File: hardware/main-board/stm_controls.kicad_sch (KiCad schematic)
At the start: 24 parts, among them SW1 SW_SPST, U1 74HC164, U10 MT8816AF1, U11 MT8816AF1, U12 MT8816AF1, U13 AD5263BRUZ200, U14 AD5263BRUZ200, U15 AD5263BRUZ200, U16 AD5263BRUZ200, U17 AD5263BRUZ200, U18 AD5263BRUZ200, U19 AD5263BRUZ200, U2 74HC164, U20 AD5263BRUZ200, U22 STM32F091RCTx, U23 FT232RL, U3 74HC164, U4 MT8816AF1, U5 MT8816AF1, U6 MT8816AF1, U7 MT8816AF1, U8 MT8816AF1, U9 MT8816AF1

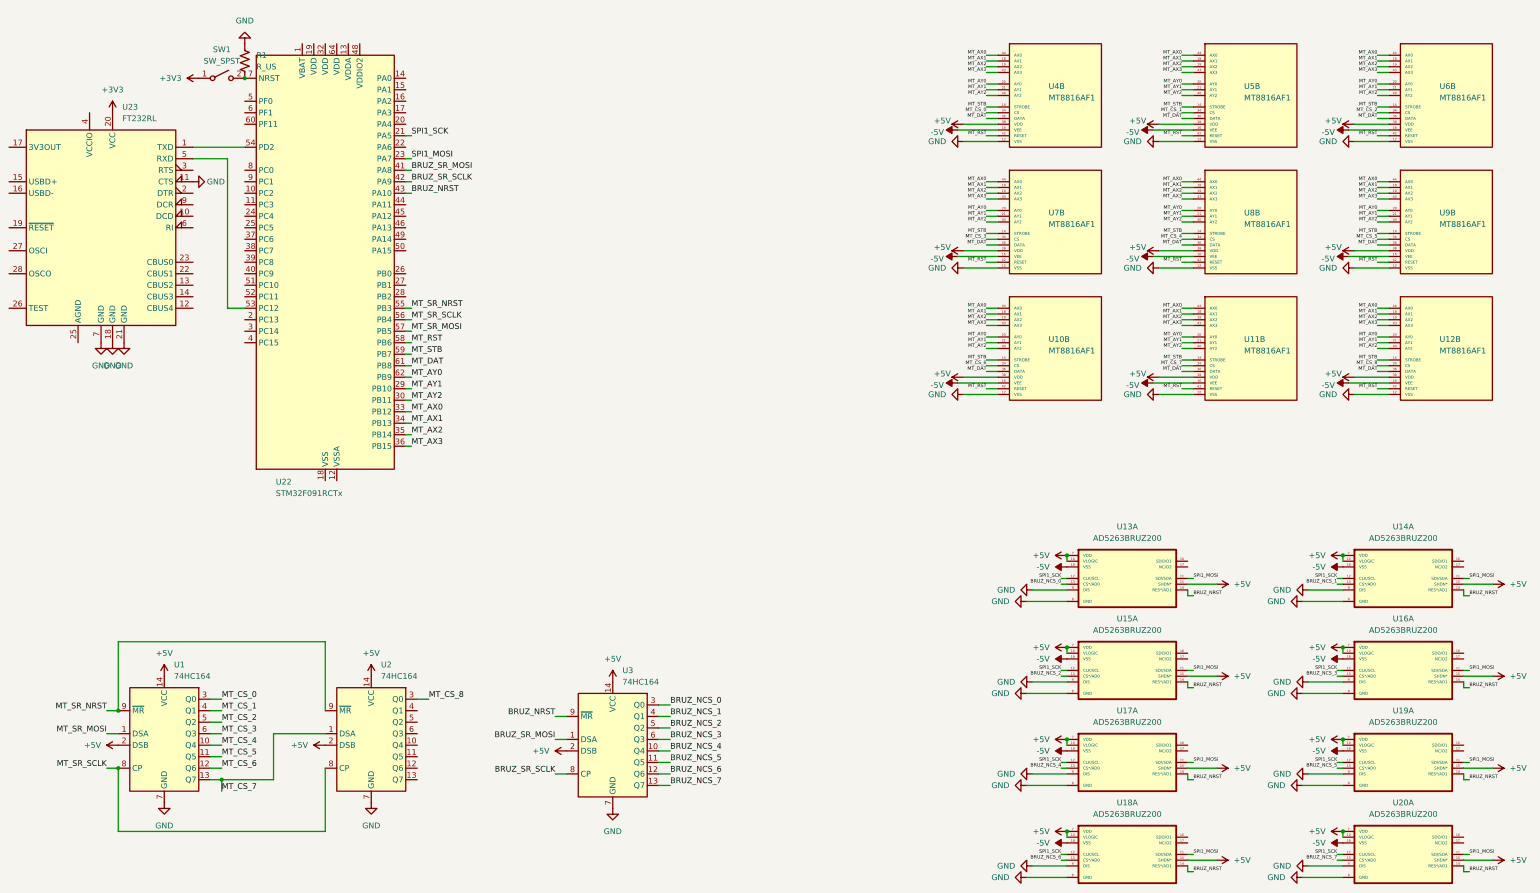
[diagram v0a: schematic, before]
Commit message: God is Real, God is Real, Im not kidding this time I wouldn't joke about this
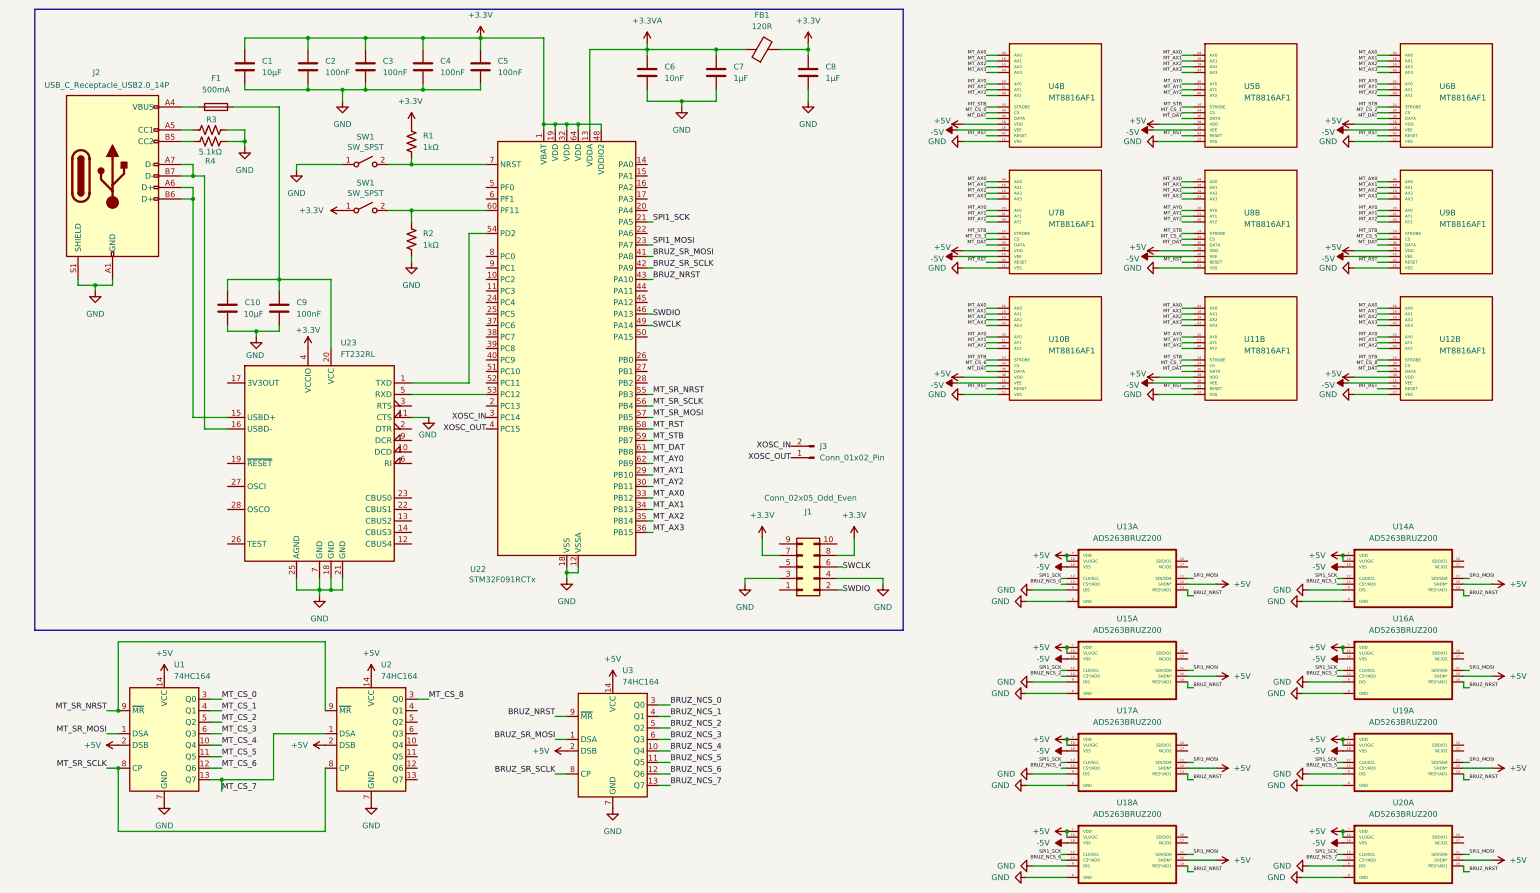
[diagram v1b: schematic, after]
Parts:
- added C1, C10: 10µF, symbol Device:C
- added C2, C3, C4, C5, C9: 100nF, symbol Device:C
- added C6: 10nF, symbol Device:C
- added C7, C8: 1µF, symbol Device:C
- added F1: 500mA, symbol Device:Fuse
- added FB1: 120R, symbol Device:FerriteBead
- added J1: Conn_02x05_Odd_Even, symbol Connector_Generic:Conn_02x05_Odd_Even
- added J2: USB_C_Receptacle_USB2.0_14P, symbol Connector:USB_C_Receptacle_USB2.0_14P
- added J3: Conn_01x02_Pin, symbol Connector:Conn_01x02_Pin
- added R2: 1kΩ, symbol Device:R_US
- added R3: 5.1kΩ, symbol Device:R_US
- added R4: R_US, symbol Device:R_US
- added SW1: SW_SPST, symbol Switch:SW_SPST
- R1: value R_US -> 1kΩ
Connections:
- net GND: now also SW1.1 (A), U22.12 (VSSA), U22.18 (VSS), U22.31 (VSS), U22.47 (VSS), U22.63 (VSS), U23.25 (AGND), C1.2, C10.2, C2.2, C3.2, C4.2, C5.2, C6.2, C7.2, C8.2, C9.2, J1.3 (Pin_3), J1.4 (Pin_4), J2.A1 (GND), J2.A12 (GND), J2.B1 (GND), J2.B12 (GND), J2.S1 (SHIELD), R2.2, R3.2, R4.2; no longer R1.1
- net at U23.15 (USBD+): now also J2.A6 (D+), J2.B6 (D+)
- net at U23.16 (USBD-): now also J2.A7 (D-), J2.B7 (D-)
- net +3.3V: now reaches U23.4 (VCCIO)
- net +3.3V: now also R1.1, U22.1 (VBAT), U22.19 (VDD), U22.32 (VDD), U22.48 (VDDIO2), U22.64 (VDD), C1.1, C2.1, C3.1, C4.1, C5.1, C8.1, FB1.2, J1.7 (Pin_7), J1.8 (Pin_8), SW1.1 (A)
- net +3.3VA: now reaches U22.13 (VDDA)
- net +3.3VA: now also C6.1, C7.1, FB1.1
- net XOSC_IN: now reaches U22.3 (PC14)
- net XOSC_IN: now also J3.2 (Pin_2)
- net XOSC_OUT: now reaches U22.4 (PC15)
- net XOSC_OUT: now also J3.1 (Pin_1)
- net SWDIO: now reaches U22.46 (PA13)
- net SWDIO: now also J1.2 (Pin_2)
- net SWCLK: now reaches U22.49 (PA14)
- net SWCLK: now also J1.6 (Pin_6)
- net at U22.60 (PF11): now also R2.1, SW1.2 (B)
- net +3V3: no longer names the net of U23.20 (VCC)
- net +3V3: now also C10.1, C9.1, F1.2; no longer SW1.1 (A)
- new net: J2.A5 (CC1), R3.1
- new net: J2.B5 (CC2), R4.1
- new net: F1.1, J2.A4 (VBUS), J2.A9 (VBUS), J2.B4 (VBUS), J2.B9 (VBUS)
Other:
- moved on the sheet: SW1, U22, U23
